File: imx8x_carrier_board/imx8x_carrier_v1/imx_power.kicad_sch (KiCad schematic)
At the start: 1 part, among them CN1 DF11-16DP-2DSA(08)

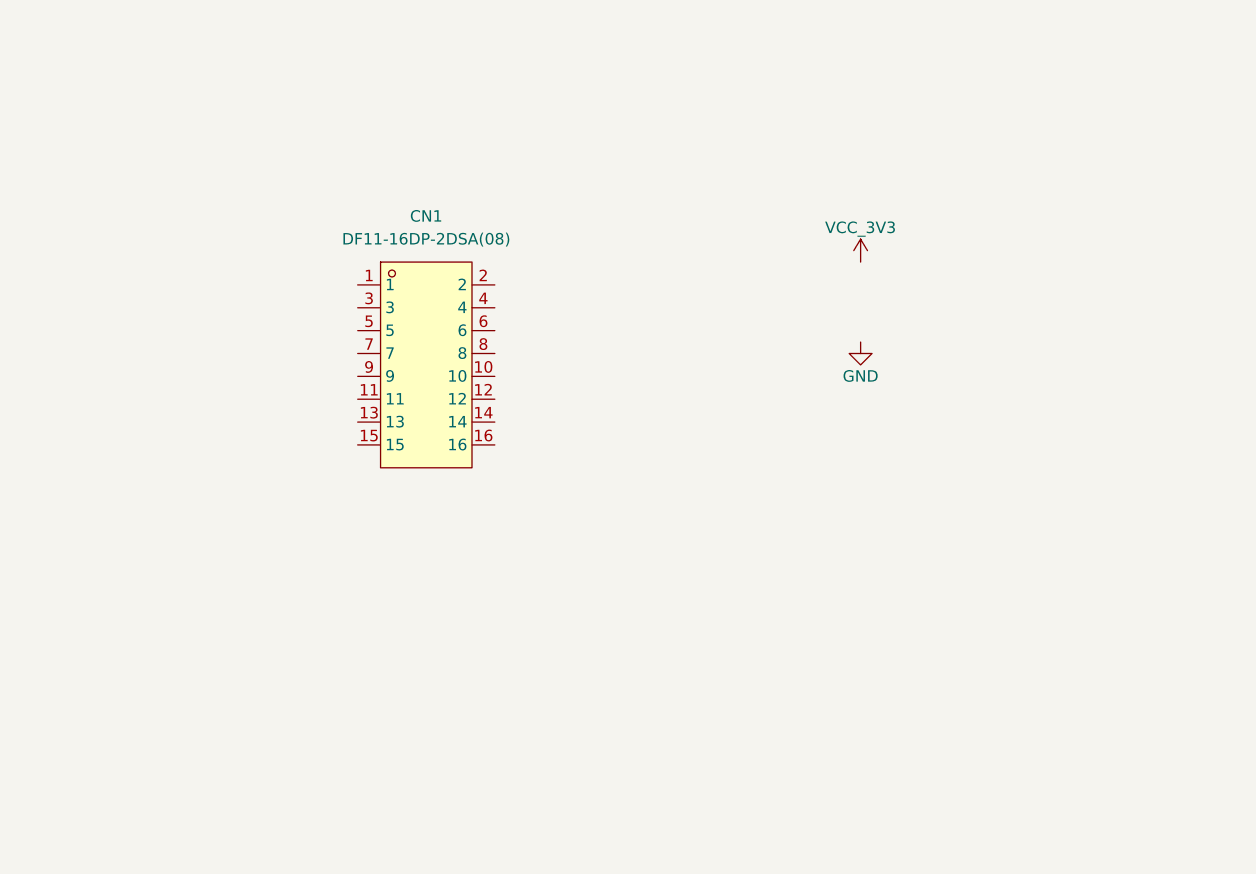
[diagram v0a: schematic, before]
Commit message: Schematic Updates
WIP.
SOM Connector global labels have been updated.
Commit to update remote. Disregard.
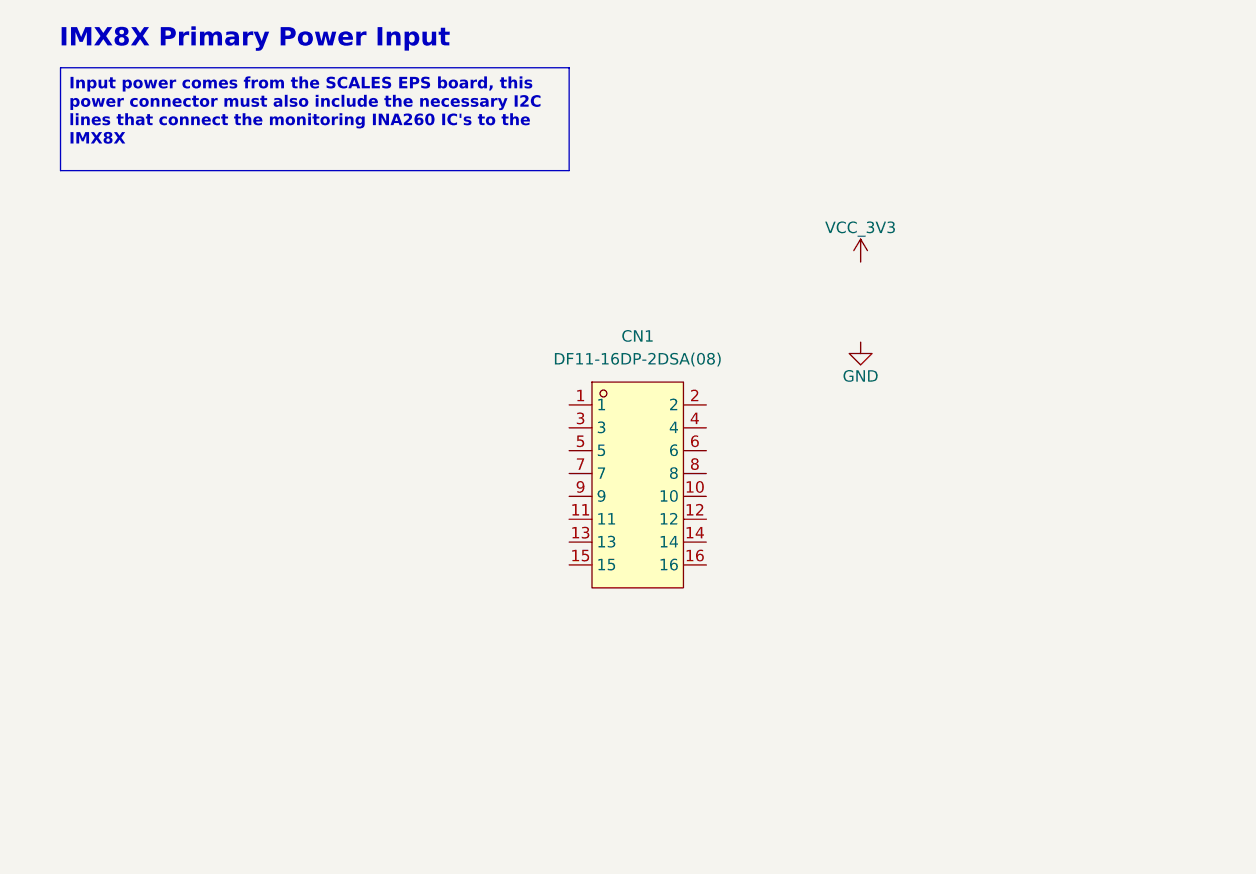
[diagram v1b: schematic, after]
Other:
- note added: "IMX8X Primary Power Input"
- moved on the sheet: CN1
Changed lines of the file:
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@@
 	(generator_version "9.0")
 	(paper "A4")
+	(text "IMX8X Primary Power Input"
+		(exclude_from_sim no)
+		(at 35.56 15.875 0)
+		(effects
+			(font
+				(size 2.032 2.032)
+				(thickness 0.4064)
+				(bold yes)
+			)
+		)
+	)
+	(text_box "Input power comes from the SCALES EPS board, this power connector must also include the necessary I2C lines that connect the monitoring INA260 IC's to the IMX8X"
+		(exclude_from_sim no)
+		(at 13.97 19.05 0)
+		(size 56.515 11.43)
+		(margins 0.9525 0.9525 0.9525 0.9525)
+		(stroke
+			(width 0)
+			(type solid)
+		)
+		(fill
+			(type none)
+		)
+		(effects
+			(font
+				(size 1.27 1.27)
+				(thickness 0.254)
+				(bold yes)
+			)
+			(justify left top)
+		)
+	)
 	(symbol
 		(lib_id "power:GND")
@@
 	(symbol
 		(lib_id "imx8_carrier_board_symbol_library:DF11-16DP-2DSA(08)")
-		(at 54.61 52.07 0)
+		(at 78.105 65.405 0)
 		(unit 1)
 		(exclude_from_sim no)
@@
 		(fields_autoplaced yes)
 		(property "Reference" "CN1"
-			(at 54.61 35.56 0)
+			(at 78.105 48.895 0)
 			(effects
 				(font
@@
 		)
 		(property "Value" "DF11-16DP-2DSA(08)"
-			(at 54.61 38.1 0)
+			(at 78.105 51.435 0)
 			(effects
 				(font
@@
 		)
 		(property "Footprint" "imx8_carrier_board_footprints:CONN-TH_DF11-16DP-2DSA-08"
-			(at 54.61 68.58 0)
+			(at 78.105 81.915 0)
 			(effects
 				(font
@@
 		)
 		(property "Datasheet" "https://lcsc.com/product-detail/Wire-To-Board-Wire-To-Wire-Connector_HRS-Hirose-HRS-DF11-16DP-2DSA-08_C530981.html"
-			(at 54.61 71.12 0)
+			(at 78.105 84.455 0)
 			(effects
 				(font
@@
 		)
 		(property "Description" ""
-			(at 54.61 52.07 0)
+			(at 78.105 65.405 0)
 			(effects
 				(font
@@
 		)
 		(property "LCSC Part" "C530981"
-			(at 54.61 73.66 0)
-			(effects
-				(font
+			(at 78.105 86.995 0)
+			(effects
+				(font

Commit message: Updated Schematic
Working on Micro SD card connector.
Working on implementing power connector. Still uncertain about some things I still need to implement. WIP
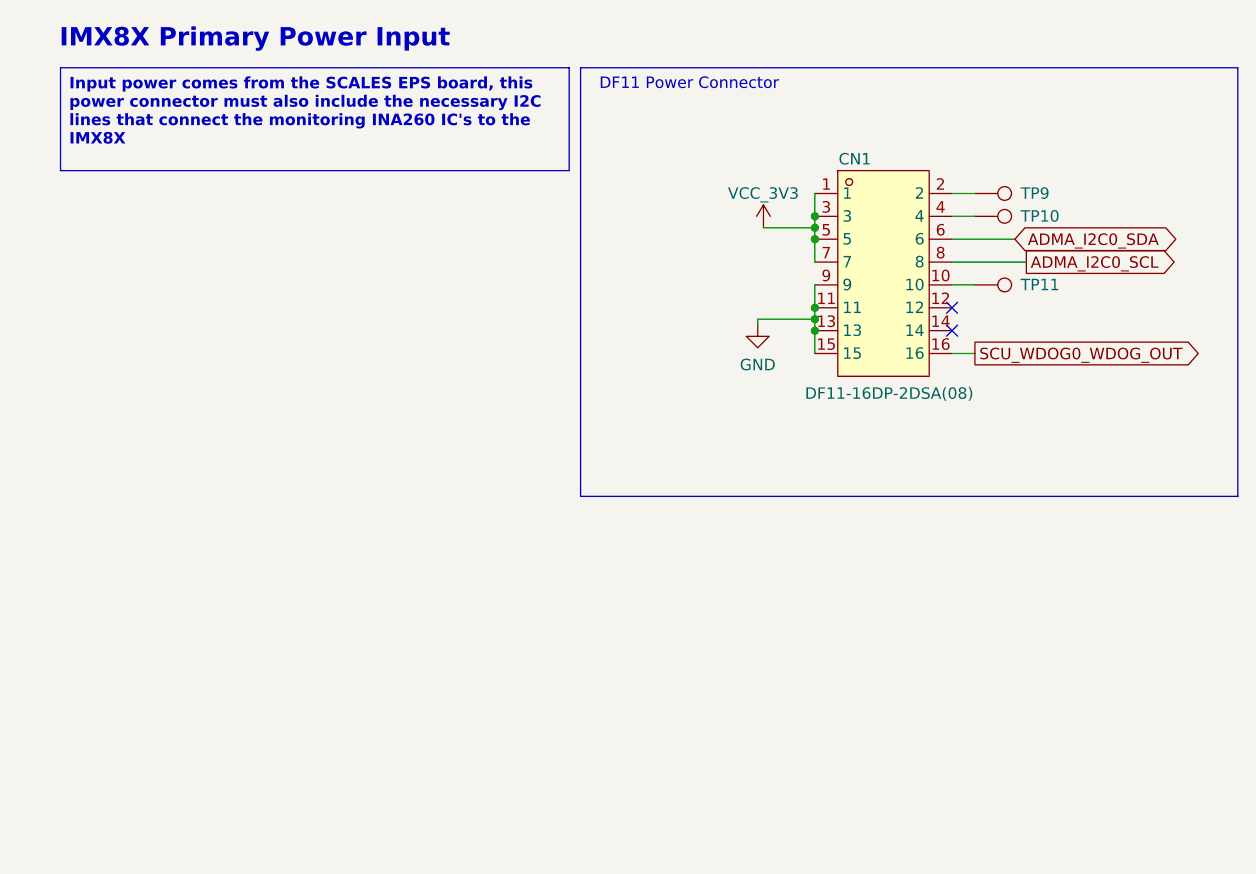
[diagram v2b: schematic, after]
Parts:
- added TP10, TP11, TP9: TestPoint, symbol Connector:TestPoint
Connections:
- net GND: now also CN1.11, CN1.13, CN1.15, CN1.9
- net VCC_3V3: now also CN1.1, CN1.3, CN1.5, CN1.7
- net at CN1.10: now also TP11.1
- net SCU_WDOG0_WDOG_OUT: now reaches CN1.16
- net at CN1.2: now also TP9.1
- net at CN1.4: now also TP10.1
- net ADMA_I2C0_SDA: now reaches CN1.6
- net ADMA_I2C0_SCL: now reaches CN1.8
- no-connect marks 0 -> 2
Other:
- note added: "DF11 Power Connector"
- moved on the sheet: CN1

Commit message: Schematic Updates
WIP
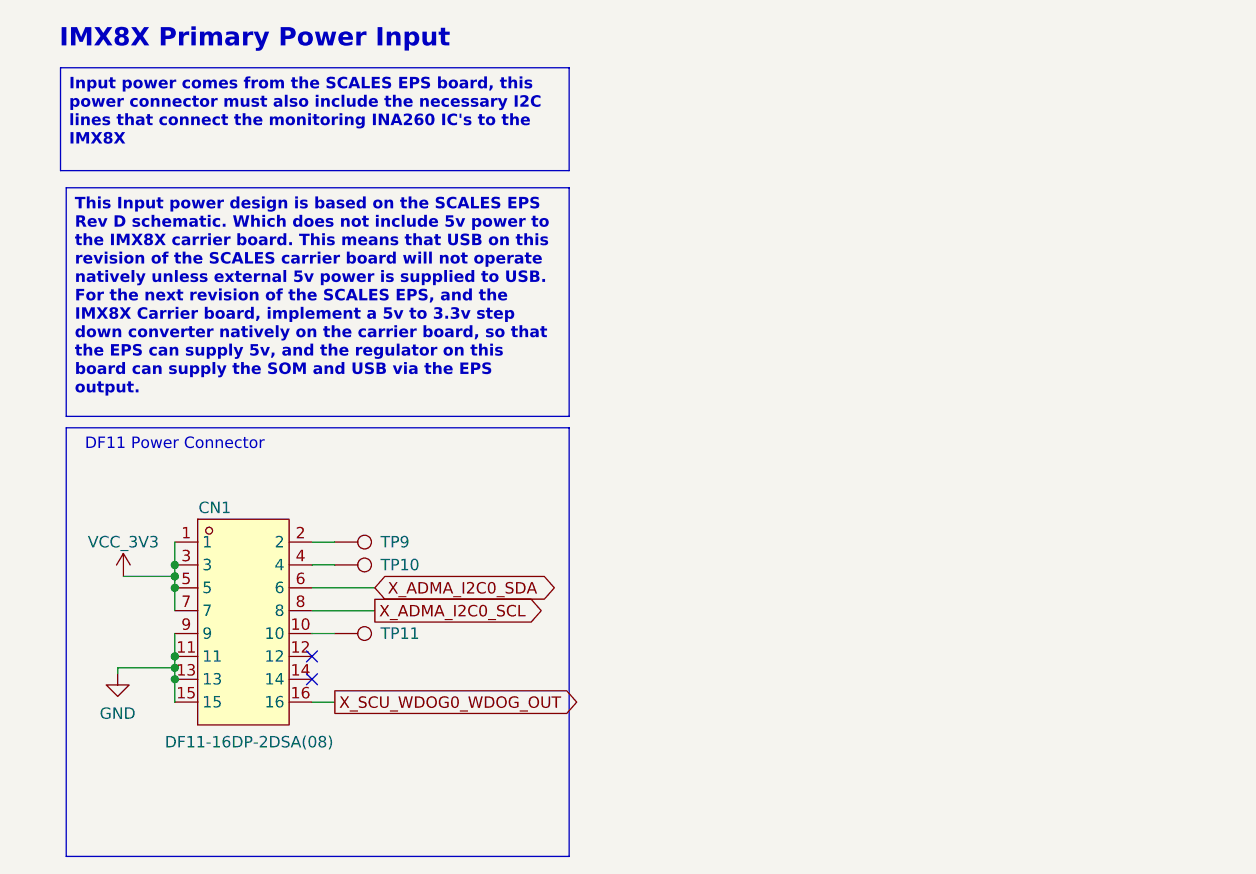
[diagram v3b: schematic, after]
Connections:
- net ADMA_I2C0_SCL renamed X_ADMA_I2C0_SCL
- net ADMA_I2C0_SDA renamed X_ADMA_I2C0_SDA
- net SCU_WDOG0_WDOG_OUT renamed X_SCU_WDOG0_WDOG_OUT
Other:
- moved on the sheet: CN1, TP10, TP11, TP9

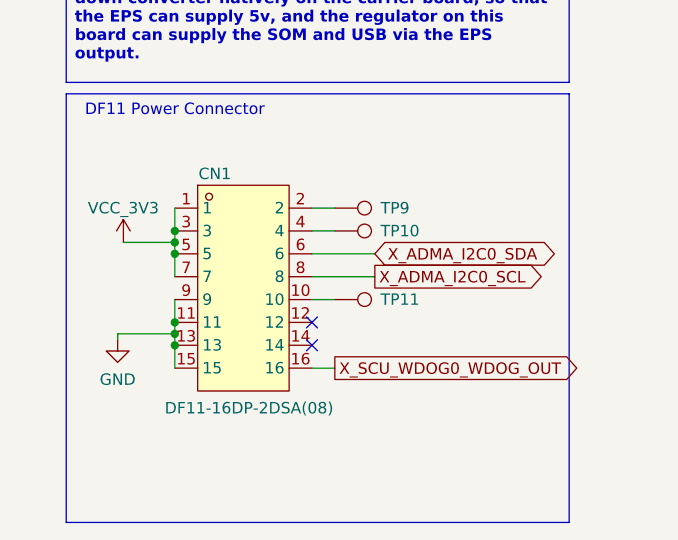
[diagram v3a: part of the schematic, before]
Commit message: Schematic Updates
WIP
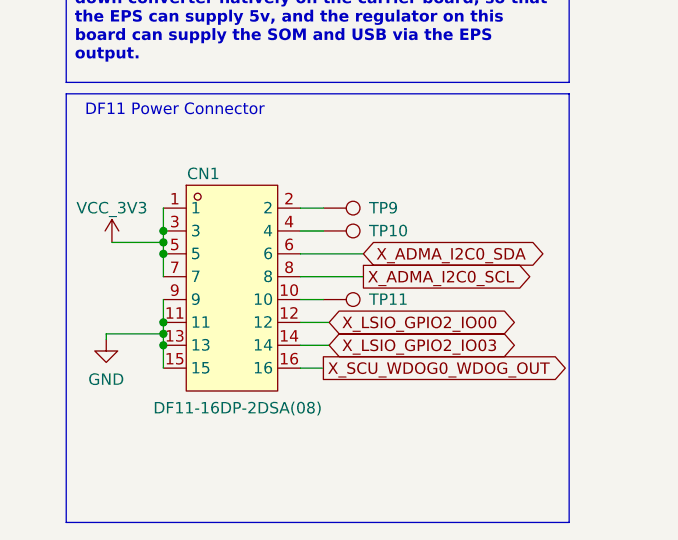
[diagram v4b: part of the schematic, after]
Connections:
- net X_LSIO_GPIO2_IO00: now reaches CN1.12
- net X_LSIO_GPIO2_IO03: now reaches CN1.14
- no-connect marks 2 -> 0
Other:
- moved on the sheet: CN1, TP10, TP11, TP9
